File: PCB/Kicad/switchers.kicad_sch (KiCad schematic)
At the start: 44 parts, among them SW1 SWPADL1, SW10 SWPADR2, SW11 SWPADR3, SW12 SWPADR4, SW13 SWPADR5, SW14 SWPADR6, SW15 SWPADR7, SW16 SWPADR8, SW17 SWPLAYL, SW18 SWCUEL, SW19 SWSHIFTL, SW2 SWPADL2, SW20 SWSYNCL, SW21 SWRANGEL, SW22 SWFX1L, SW23 SWFX2L, SW24 SWFX3L, SW25 SWBR-PREVL, SW26 SWBR-BACKL, SW27 SWPLAYR, SW28 SWCUER, SW29 SWSHIFTR, SW3 SWPADL3, SW30 SWSYNCR, SW31 SWRANGER, SW32 SWFX1R, SW33 SWFX2R, SW34 SWFX3R, SW35 SWBR-PREVR, SW36 SWBR-BACKR, SW37 SWPCUEL1, SW38 SWPCUEL2, SW39 SWPCUEL3, SW4 SWPADL4, SW40 SWSEL1, SW41 SWSEL2, SW42 SWSEL3, SW43 BROWSER-L, SW44 BROWSER-R, SW5 SWPADL5, SW6 SWPADL6, SW7 SWPADL7, SW8 SWPADL8, SW9 SWPADR1

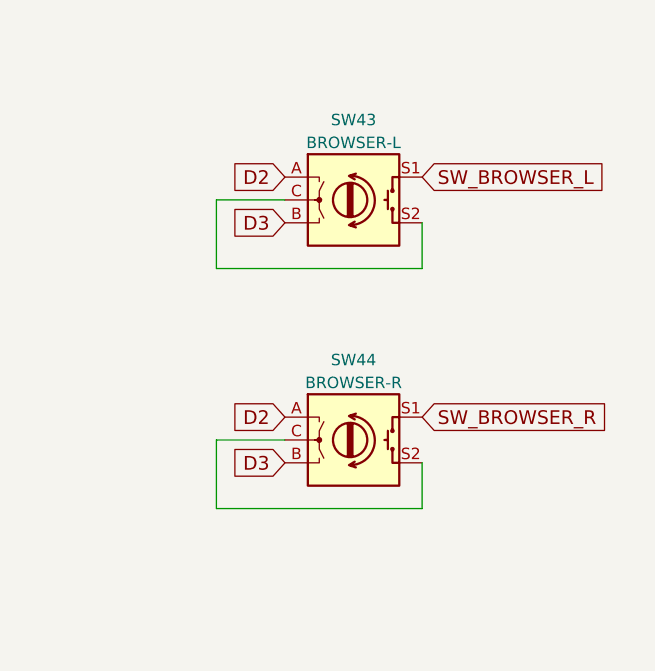
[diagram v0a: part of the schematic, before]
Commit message: trillbar added
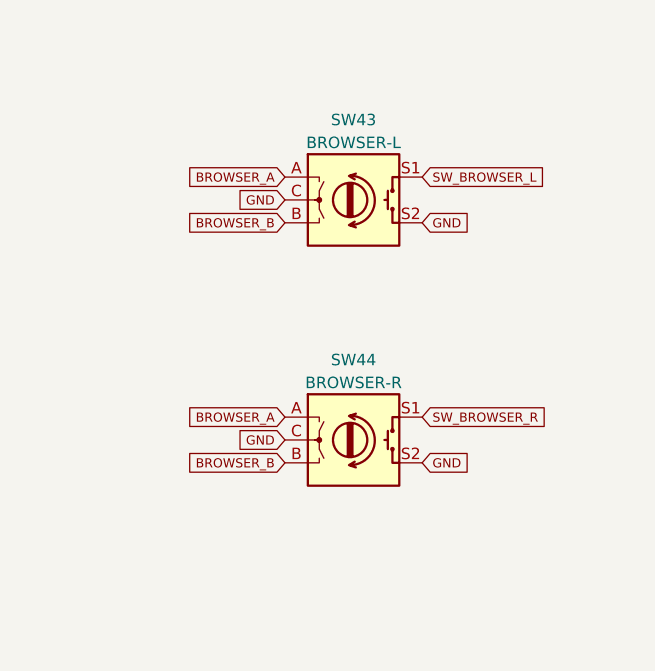
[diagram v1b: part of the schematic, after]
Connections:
- net GND: now also SW43.C, SW43.S2, SW44.C, SW44.S2
- net D2 renamed BROWSER_A
- net D3 renamed BROWSER_B
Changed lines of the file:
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@@
     (stroke (width 0) (type solid) (color 0 0 0 0))
   )
-  (wire (pts (xy 223.52 72.39) (xy 223.52 80.01))
-    (stroke (width 0) (type solid) (color 0 0 0 0))
-  )
-  (wire (pts (xy 223.52 80.01) (xy 246.38 80.01))
-    (stroke (width 0) (type solid) (color 0 0 0 0))
-  )
-  (wire (pts (xy 223.52 99.06) (xy 223.52 106.68))
-    (stroke (width 0) (type solid) (color 0 0 0 0))
-  )
-  (wire (pts (xy 223.52 106.68) (xy 246.38 106.68))
-    (stroke (width 0) (type solid) (color 0 0 0 0))
-  )
-  (wire (pts (xy 231.14 72.39) (xy 223.52 72.39))
-    (stroke (width 0) (type solid) (color 0 0 0 0))
-  )
-  (wire (pts (xy 231.14 99.06) (xy 223.52 99.06))
-    (stroke (width 0) (type solid) (color 0 0 0 0))
-  )
-  (wire (pts (xy 246.38 74.93) (xy 246.38 80.01))
-    (stroke (width 0) (type solid) (color 0 0 0 0))
-  )
-  (wire (pts (xy 246.38 101.6) (xy 246.38 106.68))
-    (stroke (width 0) (type solid) (color 0 0 0 0))
-  )
   (global_label "SWPAD-L1" (shape input) (at 40.64 33.02 0)
     (effects (font (size 1.016 1.016)) (justify left))
@@
     )
   )
-  (global_label "D2" (shape input) (at 231.14 69.85 180)
-    (effects (font (size 1.524 1.524)) (justify right))
-    (property "Intersheet References" "${INTERSHEET_REFS}" (id 0) (at 483.87 144.78 0)
-      (effects (font (size 1.27 1.27)) hide)
-    )
-  )
-  (global_label "D3" (shape input) (at 231.14 74.93 180)
-    (effects (font (size 1.524 1.524)) (justify right))
-    (property "Intersheet References" "${INTERSHEET_REFS}" (id 0) (at 1.905 -30.48 0)
-      (effects (font (size 1.27 1.27)) hide)
-    )
-  )
-  (global_label "D2" (shape input) (at 231.14 96.52 180)
-    (effects (font (size 1.524 1.524)) (justify right))
-    (property "Intersheet References" "${INTERSHEET_REFS}" (id 0) (at 483.87 171.45 0)
-      (effects (font (size 1.27 1.27)) hide)
-    )
-  )
-  (global_label "D3" (shape input) (at 231.14 101.6 180)
-    (effects (font (size 1.524 1.524)) (justify right))
-    (property "Intersheet References" "${INTERSHEET_REFS}" (id 0) (at 1.905 -3.81 0)
-      (effects (font (size 1.27 1.27)) hide)
+  (global_label "BROWSER_A" (shape input) (at 231.14 69.85 180)
+    (effects (font (size 1.016 1.016)) (justify right))
+    (property "Intersheet References" "${INTERSHEET_REFS}" (id 0) (at 220.4043 69.7865 0)
+      (effects (font (size 1.016 1.016)) (justify right) hide)
+    )
+  )
+  (global_label "GND" (shape input) (at 231.14 72.39 180)
+    (effects (font (size 1.016 1.016)) (justify right))
+    (property "Intersheet References" "${INTERSHEET_REFS}" (id 0) (at 226.1132 72.3265 0)
+      (effects (font (size 1.016 1.016)) (justify right) hide)
+    )
+  )
+  (global_label "BROWSER_B" (shape input) (at 231.14 74.93 180)
+    (effects (font (size 1.016 1.016)) (justify right))
+    (property "Intersheet References" "${INTERSHEET_REFS}" (id 0) (at 220.2591 74.8665 0)
+      (effects (font (size 1.016 1.016)) (justify right) hide)
+    )
+  )
+  (global_label "BROWSER_A" (shape input) (at 231.14 96.52 180)
+    (effects (font (size 1.016 1.016)) (justify right))
+    (property "Intersheet References" "${INTERSHEET_REFS}" (id 0) (at 220.4043 96.4565 0)
+      (effects (font (size 1.016 1.016)) (justify right) hide)
+    )
+  )
+  (global_label "GND" (shape input) (at 231.14 99.06 180)
+    (effects (font (size 1.016 1.016)) (justify right))
+    (property "Intersheet References" "${INTERSHEET_REFS}" (id 0) (at 226.1132 98.9965 0)
+      (effects (font (size 1.016 1.016)) (justify right) hide)
+    )
+  )
+  (global_label "BROWSER_B" (shape input) (at 231.14 101.6 180)
+    (effects (font (size 1.016 1.016)) (justify right))
+    (property "Intersheet References" "${INTERSHEET_REFS}" (id 0) (at 220.2591 101.5365 0)
+      (effects (font (size 1.016 1.016)) (justify right) hide)
     )
   )
   (global_label "SW_BROWSER_L" (shape input) (at 246.38 69.85 0)
-    (effects (font (size 1.524 1.524)) (justify left))
-    (property "Intersheet References" "${INTERSHEET_REFS}" (id 0) (at 266.7653 69.7548 0)
-      (effects (font (size 1.524 1.524)) (justify left) hide)
+    (effects (font (size 1.016 1.016)) (justify left))
+    (property "Intersheet References" "${INTERSHEET_REFS}" (id 0) (at 259.9702 69.7865 0)
+      (effects (font (size 1.016 1.016)) (justify left) hide)
+    )
+  )
+  (global_label "GND" (shape input) (at 246.38 74.93 0)
+    (effects (font (size 1.016 1.016)) (justify left))
+    (property "Intersheet References" "${INTERSHEET_REFS}" (id 0) (at 251.4068 74.8665 0)
+      (effects (font (size 1.016 1.016)) (justify left) hide)
     )
   )
   (global_label "SW_BROWSER_R" (shape input) (at 246.38 96.52 0)
-    (effects (font (size 1.524 1.524)) (justify left))
-    (property "Intersheet References" "${INTERSHEET_REFS}" (id 0) (at 267.0556 96.4248 0)
-      (effects (font (size 1.524 1.524)) (justify left) hide)
-    )
-  )
+    (effects (font (size 1.016 1.016)) (justify left))
+    (property "Intersheet References" "${INTERSHEET_REFS}" (id 0) (at 260.1637 96.4565 0)
+      (effects (font (size 1.016 1.016)) (justify left) hide)
+    )
+  )
+  (global_label "GND" (shape input) (at 246.38 101.6 0)
+    (effects (font (size 1.016 1.016)) (justify left))
+    (property "Intersheet References" "${INTERSHEET_REFS}" (id 0) (at 251.4068 101.5365 0)
+      (effects (font (size 1.016 1.016)) (justify left) hide)
+    )
+  )
